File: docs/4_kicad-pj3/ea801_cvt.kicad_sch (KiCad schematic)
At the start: 8 parts, among them J1 Conn_01x04, J2 VL6180X, J2_BitDogLab1 J2_IDC_BitDogLab, J2_BitDogLab2 Conn_01x06_MountingPin, M1 Motor principal, M2 Motor Fuso Câmbio, U1 L293D

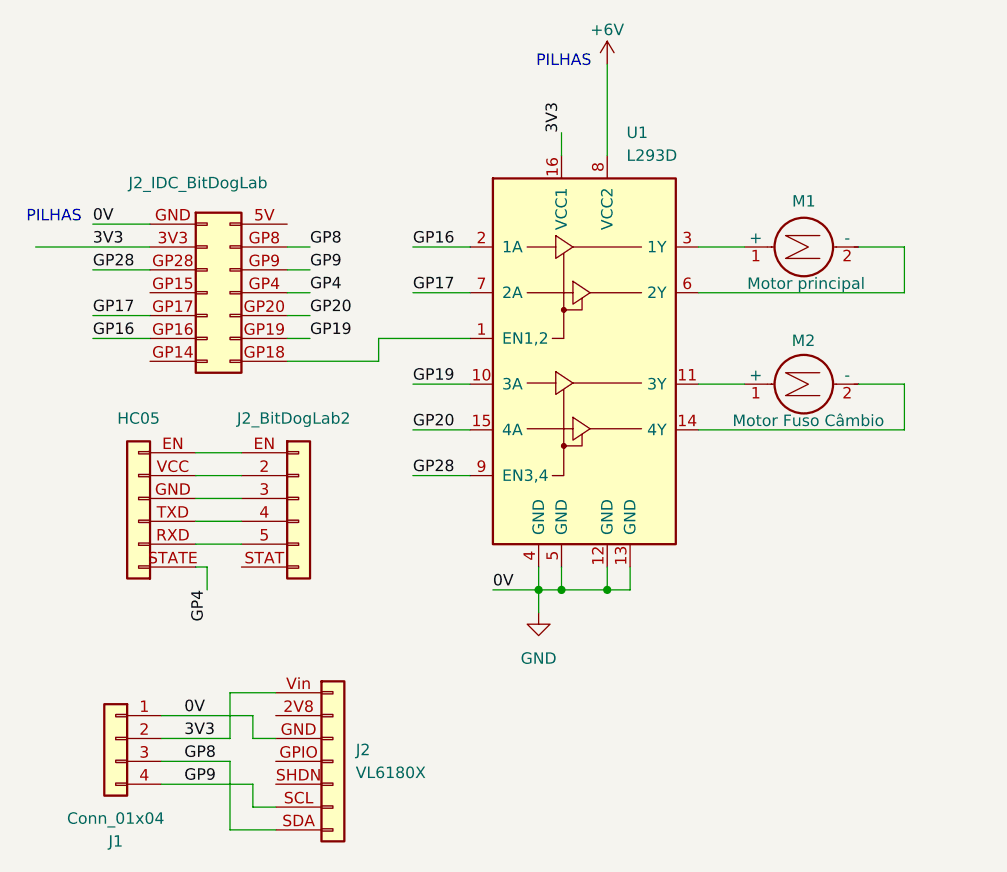
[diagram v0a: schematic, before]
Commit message: asbuilt do projeto do schematic
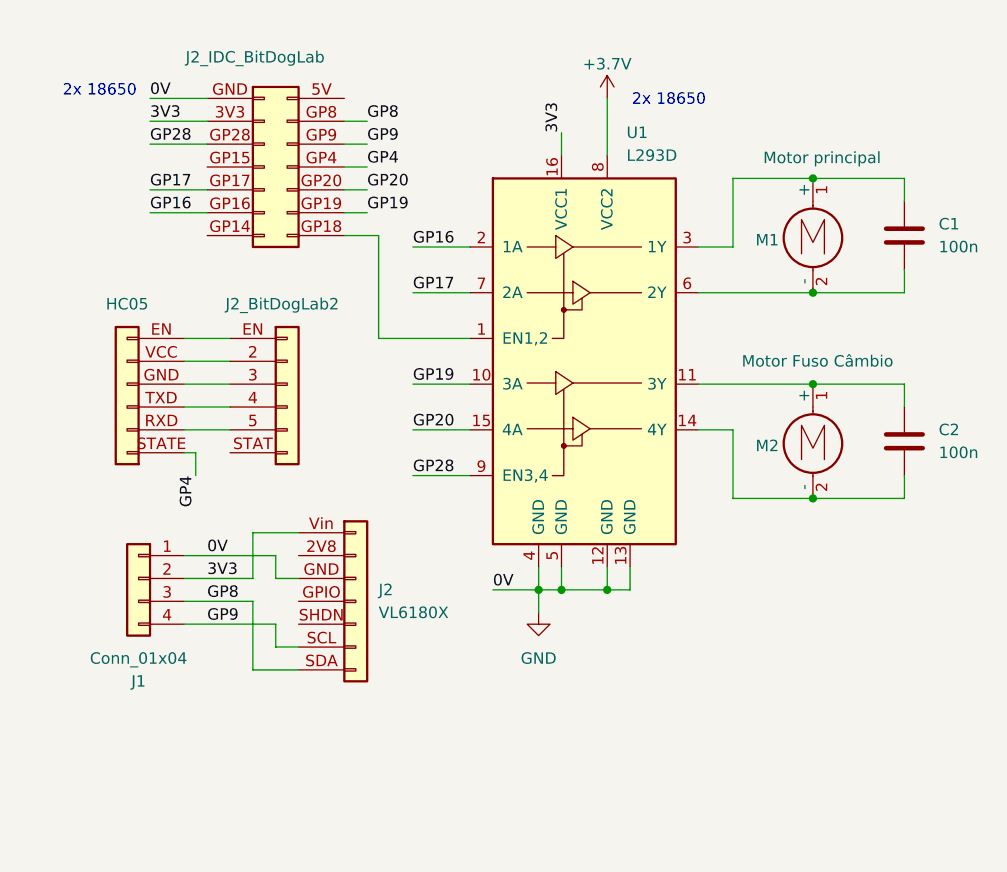
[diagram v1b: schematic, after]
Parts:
- added C1, C2: 100n, symbol Device:C
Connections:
- net at M2.1 (+), U1.11 (3Y): now also C2.1
- net at M2.2 (-), U1.14 (4Y): now also C2.2
- net at M1.1 (+), U1.3 (1Y): now also C1.1
- net at M1.2 (-), U1.6 (2Y): now also C1.2
- net +6V renamed +3.7V
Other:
- note added: "2x 18650"
- note removed: "PILHAS"
- moved on the sheet: HC05, J1, J2, J2_BitDogLab2, M1, M2
